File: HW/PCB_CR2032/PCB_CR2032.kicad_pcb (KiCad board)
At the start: 4 copper layers, 39.1 x 48 mm, 76 parts, among them J1 STDC14, J2 Breakoff, J3 PWR, M00 LED, M01 LED, M02 LED, M03 LED, M10 LED, M11 LED, M12 LED, M13 LED, SW1 WAKE, U1 STM32L071CBTx, U2 LIS3DH, Y1 32768 Hz

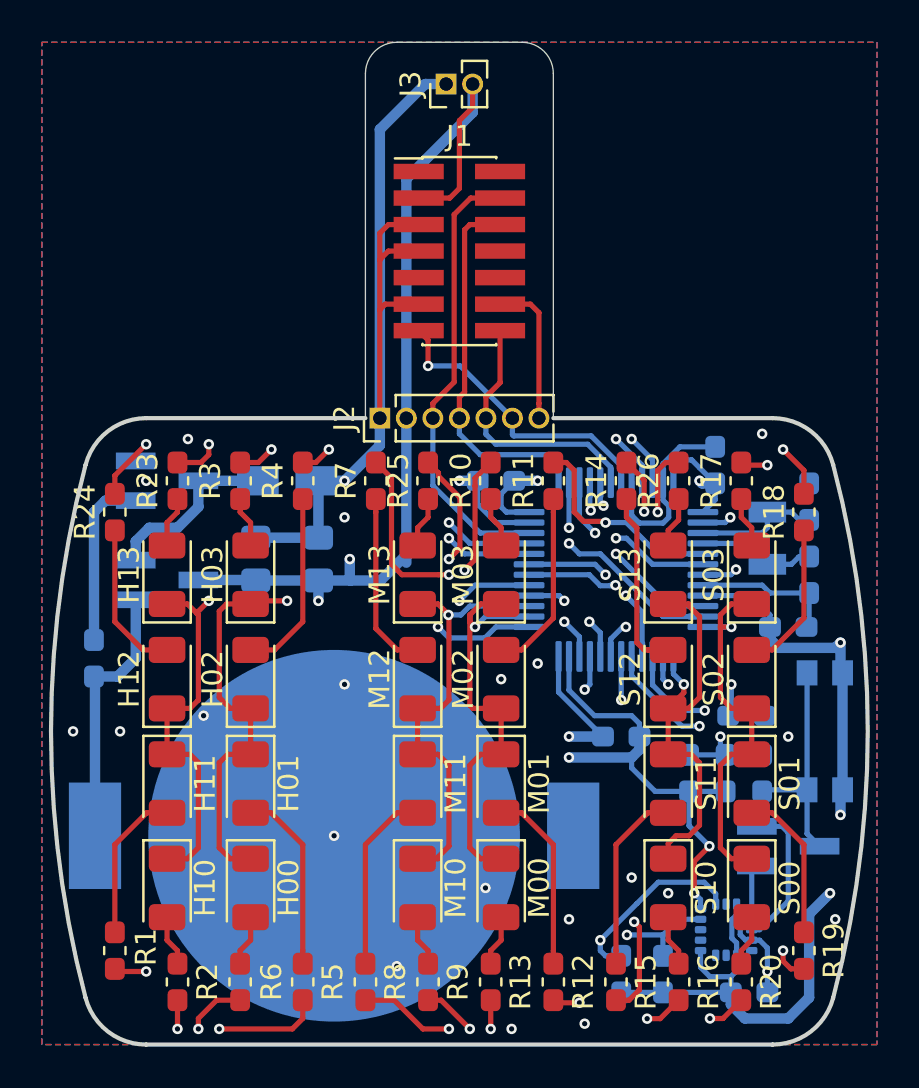
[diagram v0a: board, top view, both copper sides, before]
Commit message: Ordered V2.0 PCB
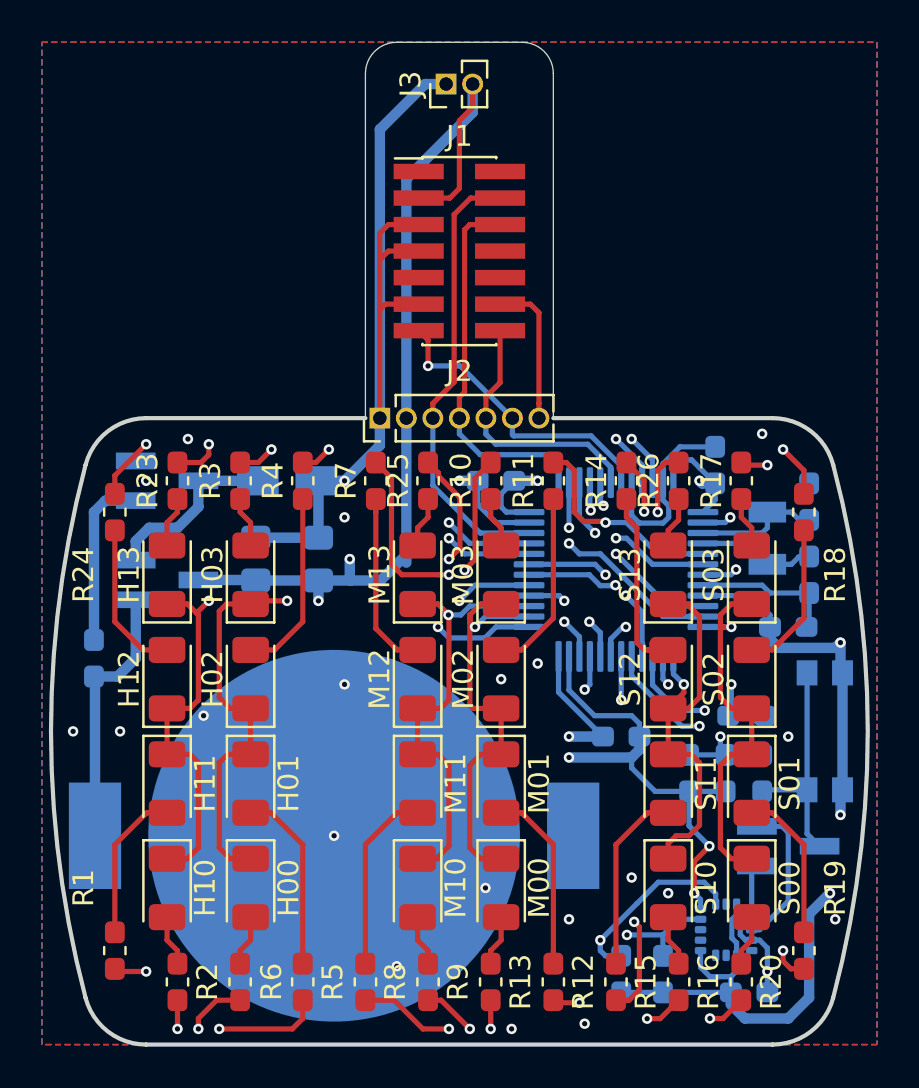
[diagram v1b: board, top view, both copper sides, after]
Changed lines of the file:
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@@
     (solder_mask_min_width 0.25)
     (aux_axis_origin 0 0)
-    (visible_elements 7FFFFFFF)
+    (visible_elements 7FFF7FFF)
     (pcbplotparams
       (layerselection 0x010fc_ffffffff)
@@
       (outputformat 1)
       (mirror false)
-      (drillshape 1)
+      (drillshape 0)
       (scaleselection 1)
-      (outputdirectory ""))
+      (outputdirectory "order_v2.0/"))
   )
   (net 0 "")
@@
     (tags "capacitor handsolder")
     (attr smd)
-    (fp_text reference C1 (at 0 1.43 90) (layer B.SilkS)
+    (fp_text reference C1 (at 1 -1.75 180) (layer B.SilkS)
       (effects (font (size 1 1) (thickness 0.15)) (justify mirror))
     )
@@
     (tags "capacitor handsolder")
     (attr smd)
-    (fp_text reference C2 (at 0 1.43 90) (layer B.SilkS)
+    (fp_text reference C2 (at 1 1.75 180) (layer B.SilkS)
       (effects (font (size 1 1) (thickness 0.15)) (justify mirror))
     )
@@
     (tags "capacitor handsolder")
     (attr smd)
-    (fp_text reference C3 (at 0 1.65 270) (layer B.SilkS)
+    (fp_text reference C3 (at -2.75 0) (layer B.SilkS)
       (effects (font (size 1 1) (thickness 0.15)) (justify mirror))
     )
@@
     (tags "capacitor handsolder")
     (attr smd)
-    (fp_text reference C5 (at 0 1.43) (layer B.SilkS)
+    (fp_text reference C5 (at -0.75 1.43) (layer B.SilkS)
       (effects (font (size 1 1) (thickness 0.15)) (justify mirror))
     )
@@
     (tags "capacitor handsolder")
     (attr smd)
-    (fp_text reference C6 (at 0 1.43 90) (layer B.SilkS)
+    (fp_text reference C6 (at 1 2 180) (layer B.SilkS)
       (effects (font (size 1 1) (thickness 0.15)) (justify mirror))
     )
@@
     (tags "capacitor handsolder")
     (attr smd)
-    (fp_text reference C9 (at 0 1.43) (layer B.SilkS)
+    (fp_text reference C9 (at 0 -1.5) (layer B.SilkS)
       (effects (font (size 1 1) (thickness 0.15)) (justify mirror))
     )
@@
     (tags "capacitor handsolder")
     (attr smd)
-    (fp_text reference C13 (at 0 1.65 270) (layer B.SilkS)
+    (fp_text reference C13 (at -2.75 0) (layer B.SilkS)
       (effects (font (size 1 1) (thickness 0.15)) (justify mirror))
     )
@@
     (tags "capacitor handsolder")
     (attr smd)
-    (fp_text reference C15 (at 0 1.43 90) (layer B.SilkS)
+    (fp_text reference C15 (at 3.25 1.75 90) (layer B.SilkS)
       (effects (font (size 1 1) (thickness 0.15)) (justify mirror))
     )
@@
     (tags "resistor handsolder")
     (attr smd)
-    (fp_text reference R1 (at -0.171267 -1.49 90) (layer F.SilkS)
+    (fp_text reference R1 (at -3 1.5 90) (layer F.SilkS)
       (effects (font (size 1 1) (thickness 0.15)))
     )
@@
     (tags "resistor handsolder")
     (attr smd)
-    (fp_text reference R18 (at 0 -1.43 90) (layer F.SilkS)
+    (fp_text reference R18 (at -3 1.5 90) (layer F.SilkS)
       (effects (font (size 1 1) (thickness 0.15)))
     )
@@
     (tags "resistor handsolder")
     (attr smd)
-    (fp_text reference R19 (at 0 -1.43 90) (layer F.SilkS)
+    (fp_text reference R19 (at -3 -1.5 90) (layer F.SilkS)
       (effects (font (size 1 1) (thickness 0.15)))
     )
@@
     (tags "resistor handsolder")
     (attr smd)
-    (fp_text reference R24 (at 0 -1.43 90) (layer F.SilkS)
+    (fp_text reference R24 (at -3 -1.5 90) (layer F.SilkS)
       (effects (font (size 1 1) (thickness 0.15)))
     )
@@
     (tags "resistor handsolder")
     (attr smd)
-    (fp_text reference R27 (at 0 1.43 90) (layer B.SilkS)
+    (fp_text reference R27 (at -3.25 0.25 90) (layer B.SilkS)
       (effects (font (size 1 1) (thickness 0.15)) (justify mirror))
     )
@@
     (tags "resistor handsolder")
     (attr smd)
-    (fp_text reference R28 (at 0 1.43 90) (layer B.SilkS)
+    (fp_text reference R28 (at 3.25 2 90) (layer B.SilkS)
       (effects (font (size 1 1) (thickness 0.15)) (justify mirror))
     )
@@
     (tags "resistor handsolder")
     (attr smd)
-    (fp_text reference R29 (at 0 1.43 90) (layer B.SilkS)
+    (fp_text reference R29 (at 3.375 0 90) (layer B.SilkS)
       (effects (font (size 1 1) (thickness 0.15)) (justify mirror))
     )
@@
     (tags "resistor handsolder")
     (attr smd)
-    (fp_text reference R30 (at 0 1.43 90) (layer B.SilkS)
+    (fp_text reference R30 (at -3.25 -2.25 90) (layer B.SilkS)
       (effects (font (size 1 1) (thickness 0.15)) (justify mirror))
     )
@@
     (tags "resistor handsolder")
     (attr smd)
-    (fp_text reference R31 (at 0 1.43 90) (layer B.SilkS)
+    (fp_text reference R31 (at 3.125 0 90) (layer B.SilkS)
       (effects (font (size 1 1) (thickness 0.15)) (justify mirror))
     )
@@
   (module "BCD-watch:WS-TASU SMT Tact Switch" (layer B.Cu)
     (at 167.5 100 270)
-    (fp_text reference SW1 (at 0 2.54 90) (layer B.SilkS)
+    (fp_text reference SW1 (at -5 -0.75 270) (layer B.SilkS)
       (effects (font (size 1 1) (thickness 0.15)) (justify mirror))
     )
@@
     (tags "LGA NoLead")
     (attr smd)
-    (fp_text reference U2 (at 0 2.45) (layer B.SilkS)
+    (fp_text reference U2 (at 2.725 0.75 90) (layer B.SilkS)
       (effects (font (size 1 1) (thickness 0.15)) (justify mirror))
     )
@@
   (module BCD-watch:FC-135 (layer B.Cu)
     (at 164.75 90.75 270)
-    (fp_text reference Y1 (at 0 2.54 90) (layer B.SilkS)
+    (fp_text reference Y1 (at 0 1.5 90) (layer B.SilkS)
       (effects (font (size 1 1) (thickness 0.15)) (justify mirror))
     )
@@
     (descr "Through hole straight pin header, 1x07, 1.27mm pitch, single row")
     (tags "Through hole pin header THT 1x07 1.27mm single row")
-    (fp_text reference J2 (at 0 -1.695 90) (layer F.SilkS)
+    (fp_text reference J2 (at 2.25 3.81 180) (layer F.SilkS)
       (effects (font (size 1 1) (thickness 0.15)))
     )
@@
   (module BCD-watch:BAT-HLD-001-xx-OTL (layer B.Cu)
     (at 144 105 180)
-    (fp_text reference BT1 (at -6.35 10.16) (layer B.SilkS)
-      (effects (font (size 1 1) (thickness 0.15)) (justify mirror))
-    )
+    (fp_text reference BT1 (at -6.35 10.16) (layer B.SilkS) hide
+      (effects (font (size 1 1) (thickness 0.15)) (justify mirror))
+    )
